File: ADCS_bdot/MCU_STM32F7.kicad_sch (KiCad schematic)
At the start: 25 parts, among them IC1 STM32F746ZGT6, SW1 SW_Push, Y1 ABM3-8.000MHZ-B4Y-T, Y2 CM7V-T1A-32.768kHz-7pF-10PPM-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

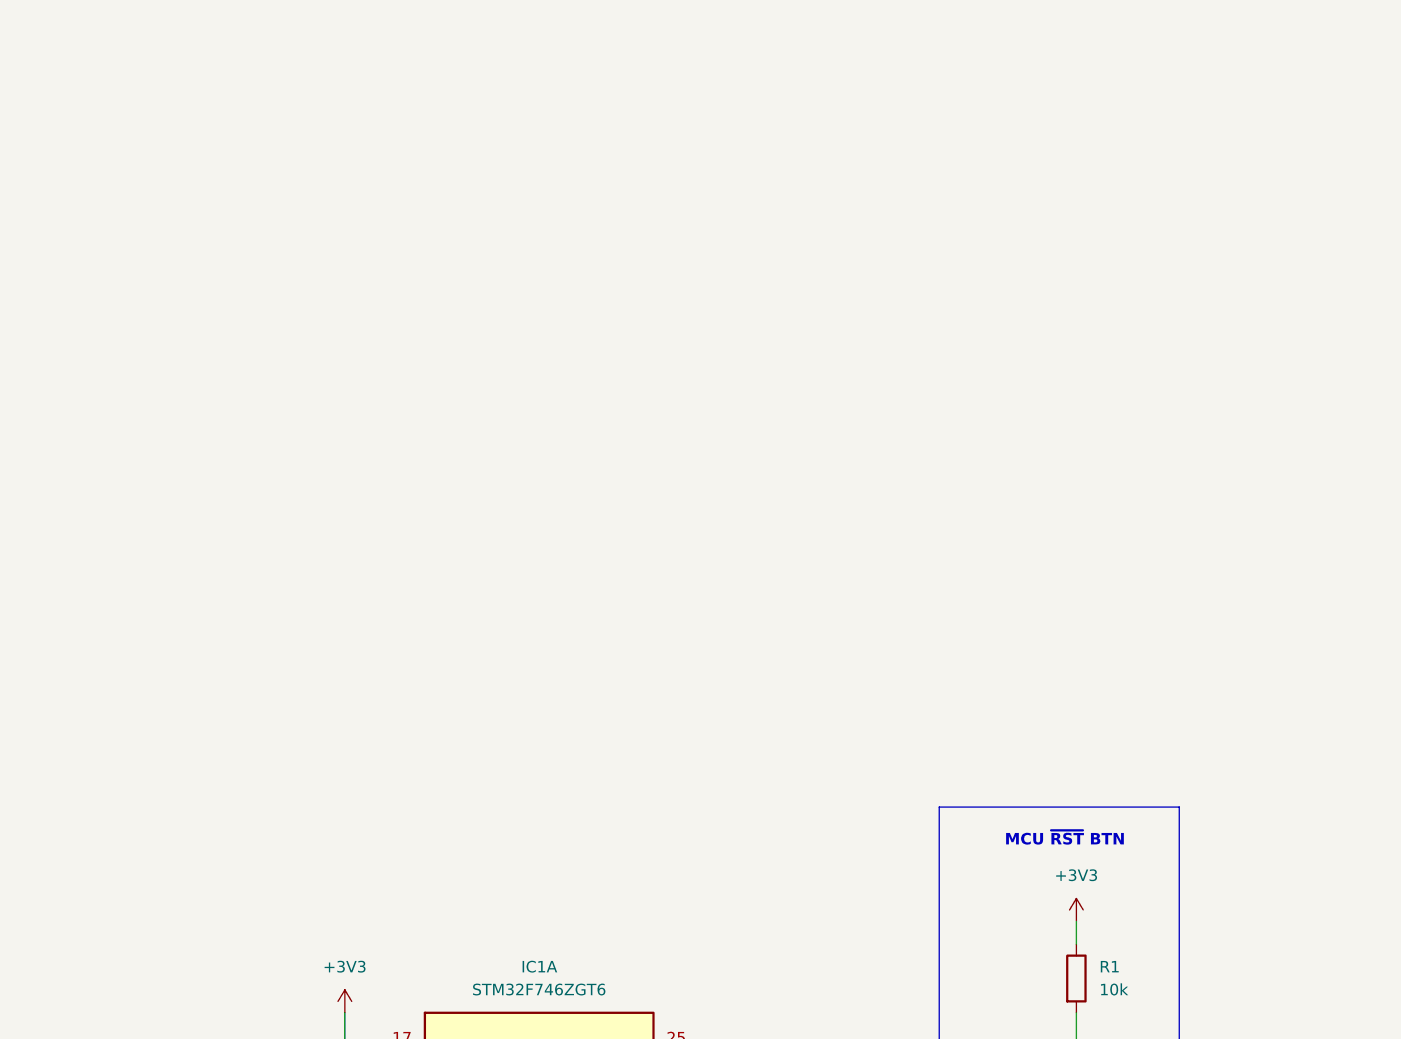
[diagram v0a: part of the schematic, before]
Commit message: add: components
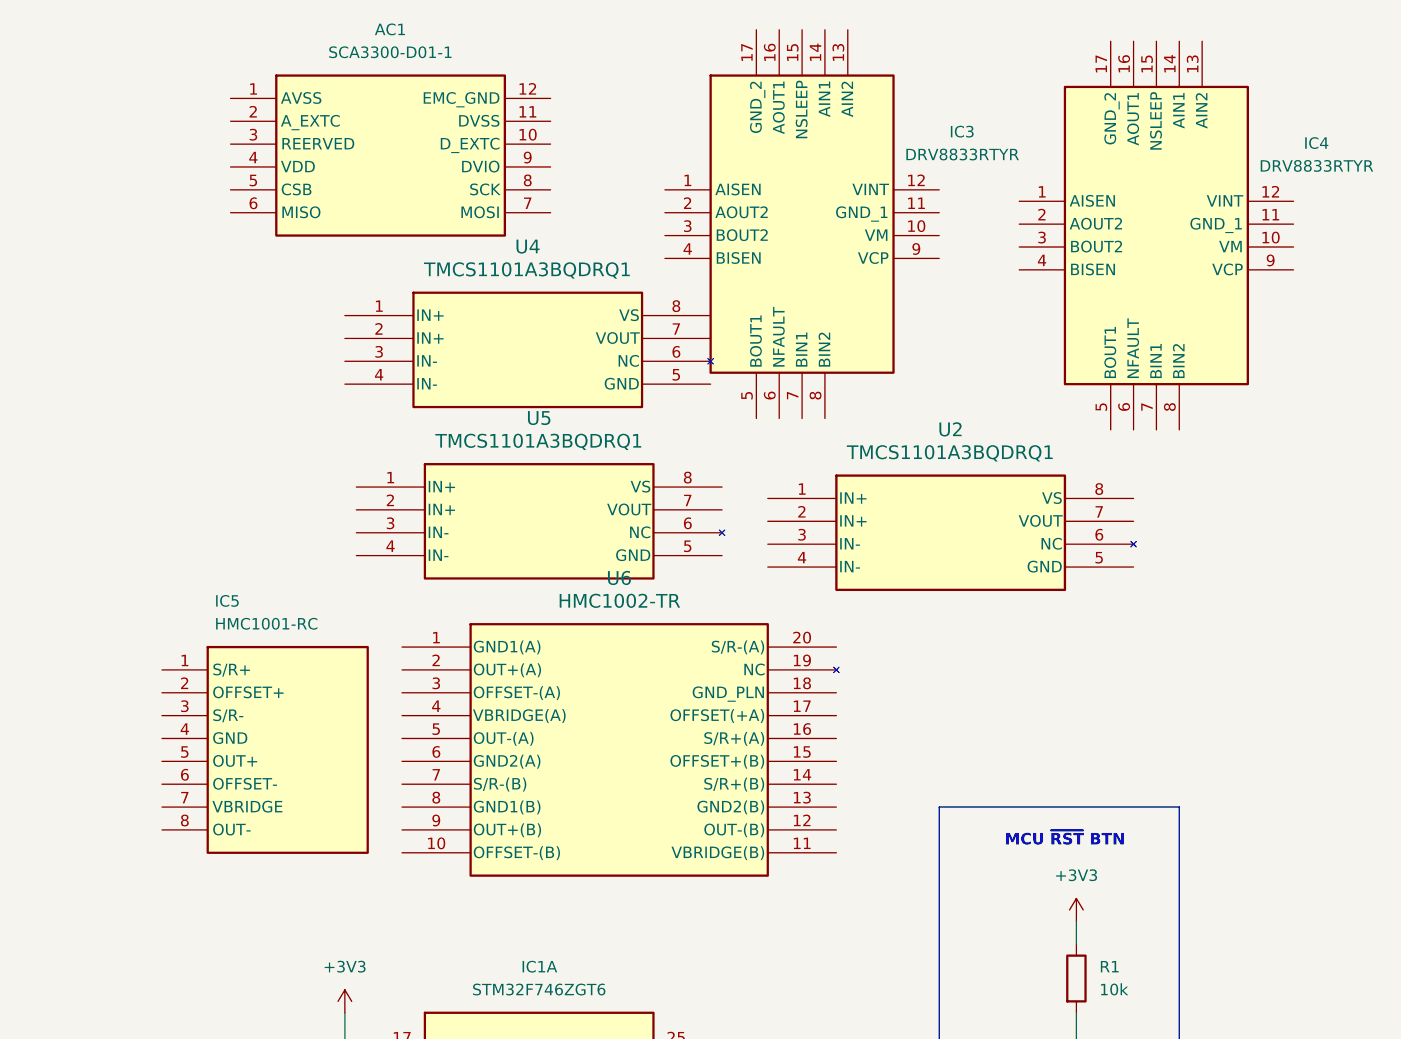
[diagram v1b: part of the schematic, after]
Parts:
- added AC1: SCA3300-D01-1, Footprintlib_adcs_bdot:SCA3300-D01-1, symbol Symbollib_adcs_bdot:SCA3300-D01-1
- added IC3, IC4: DRV8833RTYR, Footprintlib_adcs_bdot:QFN65P400X400X80-17N-D, symbol Symbollib_adcs_bdot:DRV8833RTYR
- added IC5: HMC1001-RC, Footprintlib_adcs_bdot:HMC1001RC, symbol Symbollib_adcs_bdot:HMC1001-RC
- added U2, U4, U5: TMCS1101A3BQDRQ1, Footprintlib_adcs_bdot:SOIC8_D_TEX, symbol Symbollib_adcs_bdot:TMCS1101A3BQDRQ1
- added U6: HMC1002-TR, Footprintlib_adcs_bdot:SOIC20_HNW, symbol Symbollib_adcs_bdot:HMC1002-TR
